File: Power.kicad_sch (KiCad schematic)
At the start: 38 parts, among them SW2 POWER SWITCH, U2 LM7805_TO220

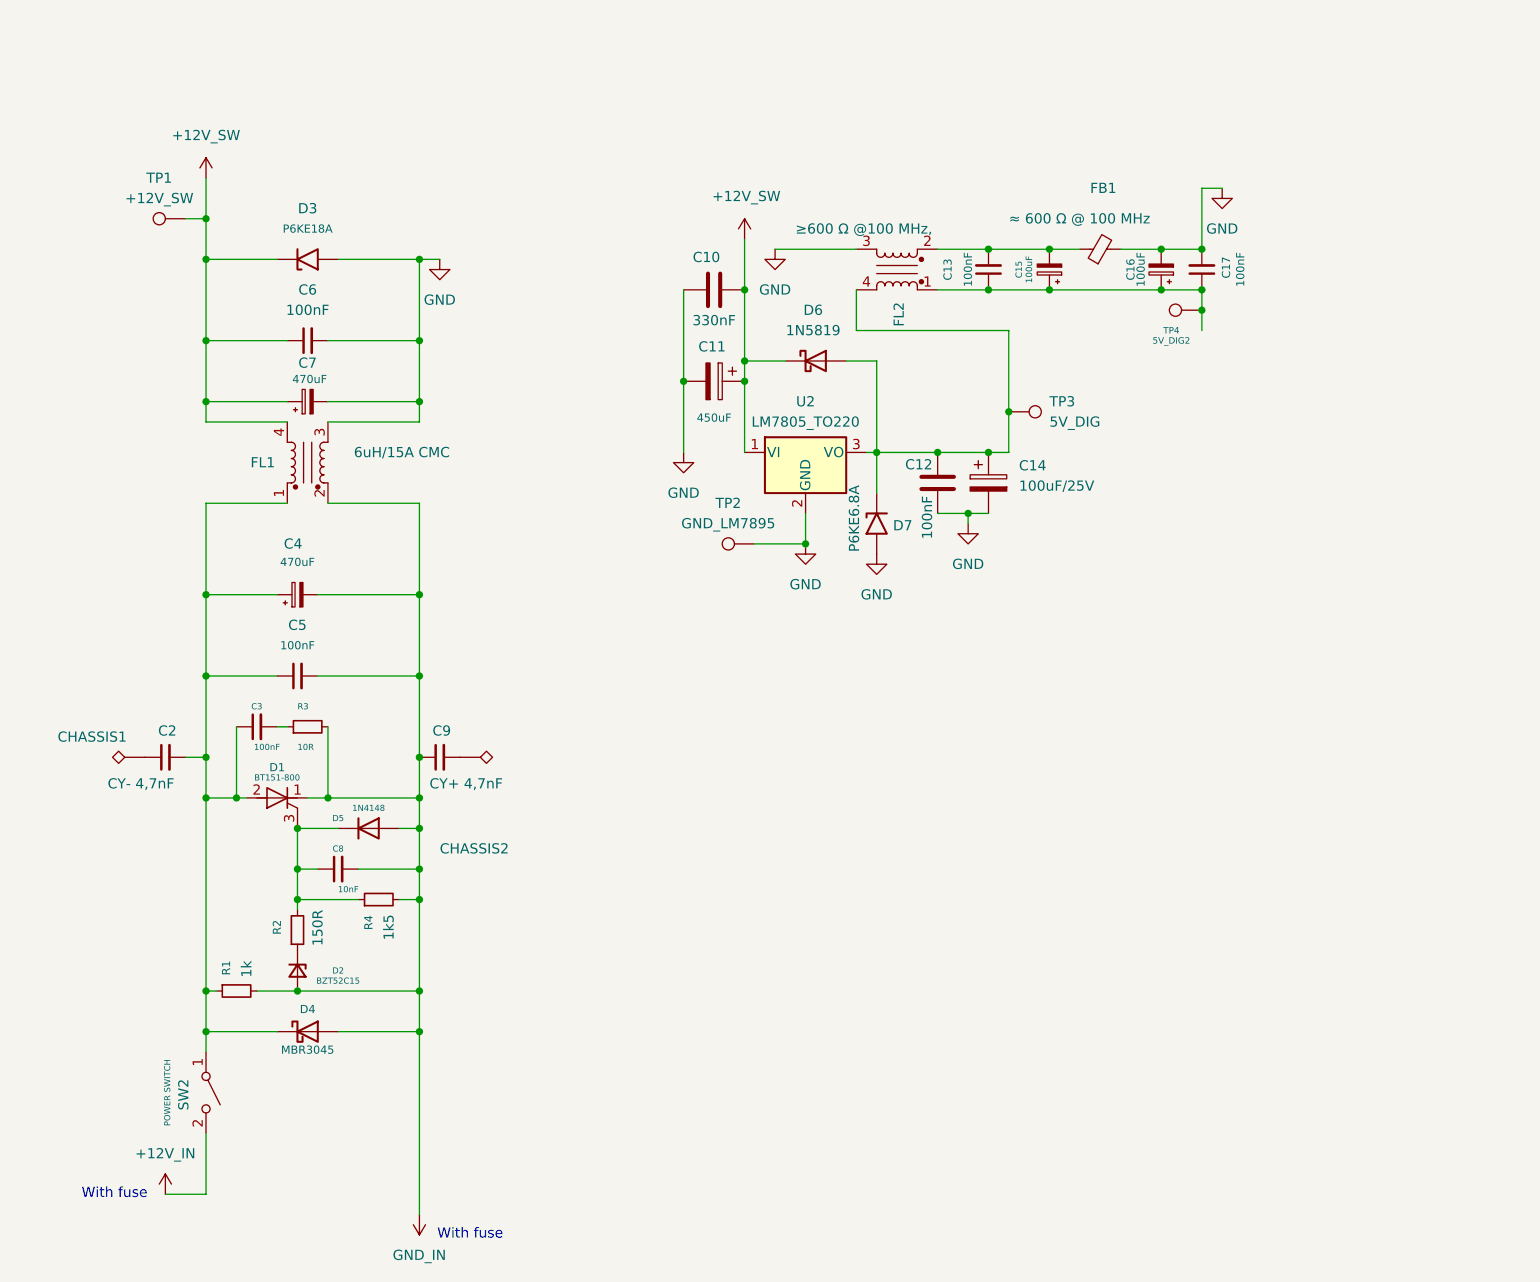
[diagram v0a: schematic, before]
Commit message: huge modification of the project.
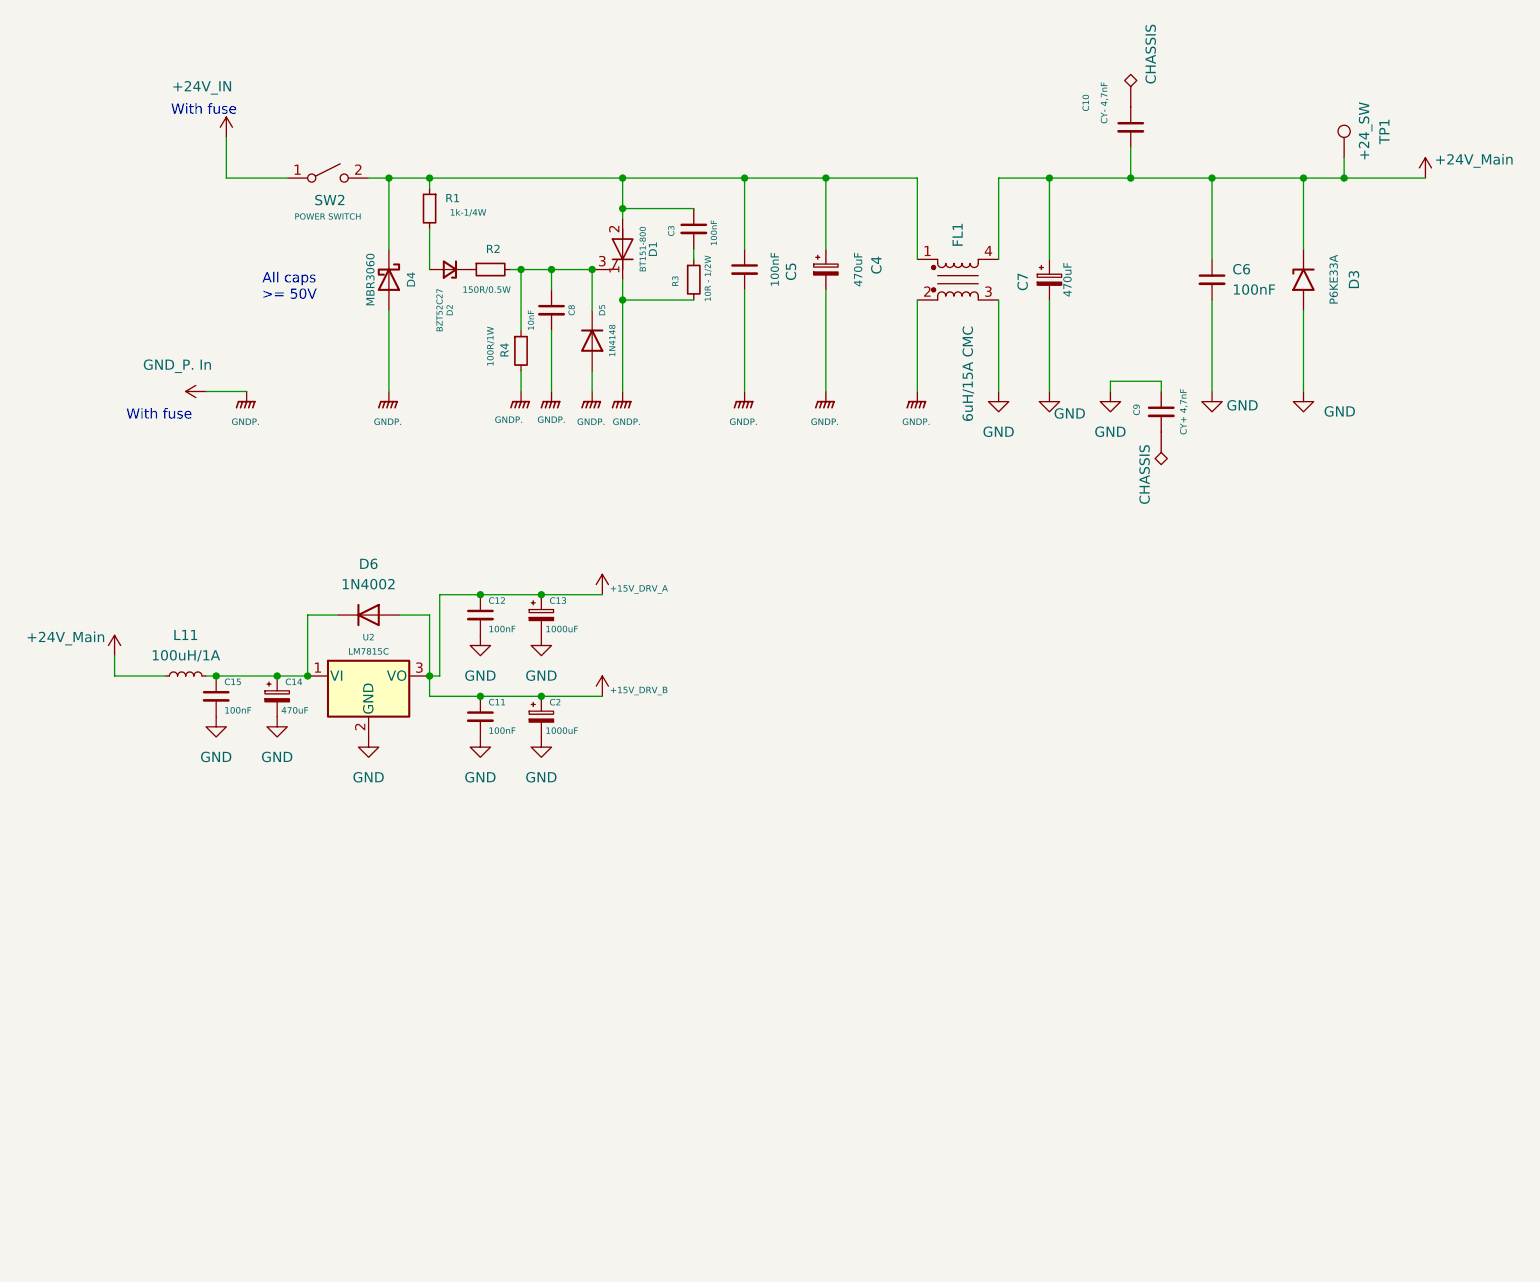
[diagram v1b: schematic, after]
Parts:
- removed C10: 330nF, symbol Device:C
- removed C11: 450uF, symbol Device:C_Polarized
- removed C12: 100nF, symbol Device:C
- removed C13, C17: 100nF, symbol Device:C_Small
- removed C14: 100uF/25V, symbol Device:C_Polarized
- removed C15, C16: 100uF, symbol Device:C_Polarized_Small
- removed C2: CY- 4,7nF, symbol Device:C_Small
- removed CHASSIS1: TestPoint_Alt, symbol Connector:TestPoint_Alt
- removed D6: 1N5819, Diode_THT:D_DO-41_SOD81_P10.16mm_Horizontal, symbol Diode:1N5819
- removed D7: P6KE6.8A, Diode_THT:D_P600_R-6_P20.00mm_Horizontal, symbol Diode:5KPxxA
- removed FB1: ≈ 600 Ω @ 100 MHz, symbol Device:FerriteBead_Small
- removed FL2: ≥600 Ω @100 MHz,, Inductor_THT:L_CommonMode_PulseElectronics_PH9455x105NL_1, symbol Filter:Choke_CommonMode_PulseElectronics_PH9455x105NL
- removed TP2: GND_LM7895, symbol Connector:TestPoint
- removed TP3: 5V_DIG, symbol Connector:TestPoint
- removed TP4: 5V_DIG2, symbol Connector:TestPoint
- removed U2: LM7805_TO220, Package_TO_SOT_THT:TO-220-3_Vertical, symbol Regulator_Linear:LM7805_TO220
- added C10: CY- 4,7nF, symbol Device:C_Small
- added C11, C12, C15: 100nF, symbol Device:C_Small
- added C13, C2: 1000uF, symbol Device:C_Polarized_Small
- added C14: 470uF, symbol Device:C_Polarized_Small
- added CHASSIS: TestPoint_Alt, symbol Connector:TestPoint_Alt
- added D6: 1N4002, Diode_THT:D_DO-41_SOD81_P10.16mm_Horizontal, symbol Diode:1N4002
- added L11: 100uH/1A, symbol Device:L_Small
- added U2: LM7815C, Package_TO_SOT_THT:TO-220-3_Vertical, symbol Regulator_Linear:LM7815_TO220
- D2: value BZT52C15 -> BZT52C27
- D3: value P6KE18A -> P6KE33A
- D4: value MBR3045 -> MBR3060
- R1: value 1k -> 1k-1/4W
- R2: value 150R -> 150R/0.5W
- R3: value 10R -> 10R - 1/2W
- R4: value 1k5 -> 100R/1W
- TP1: value +12V_SW -> +24_SW
- renumbered CHASSIS2 to CHASSIS
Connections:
- net +12V_IN is gone; now on an unnamed net: SW2.2 (B)
- net GND: now also C9.1, C11.2, C12.2, C13.2, C14.2, C15.2, C2.2, U2.2 (GND)
- net at C3.1, C4.1, C5.1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: no longer SW2.1 (A)
- net +12V_SW renamed +24V_Main
- net +24V_Main: now also C10.2, L11.1
- net GND_IN renamed GNDP.
- net GNDP.: no longer C9.1, D2.2 (A), R1.2
- new net: D2.2 (A), R1.2
- new net: C10.1, CHASSIS.1
- new net: C14.1, C15.1, D6.1 (K), L11.2, U2.1 (VI)
- new net +15V_DRV_A: C11.1, C12.1, C13.1, C2.1, D6.2 (A), U2.3 (VO)
- new net +24V_IN: SW2.1 (A)
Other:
- note added: "All caps >= 50V"
- moved on the sheet: C3, C4, C5, C6, C7, C8, C9, CHASSIS, D1, D2, D3, D4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
